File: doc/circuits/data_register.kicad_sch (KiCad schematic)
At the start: 12 parts, among them U1 74LS193, U10 74LS32, U11 74LS32, U13 74LS193, U2 74LS00, U3 74LS245, U4 74LS00, U5 74LS00, U6 74LS32, U7 74LS245, U8 74LS32, U9 74LS32

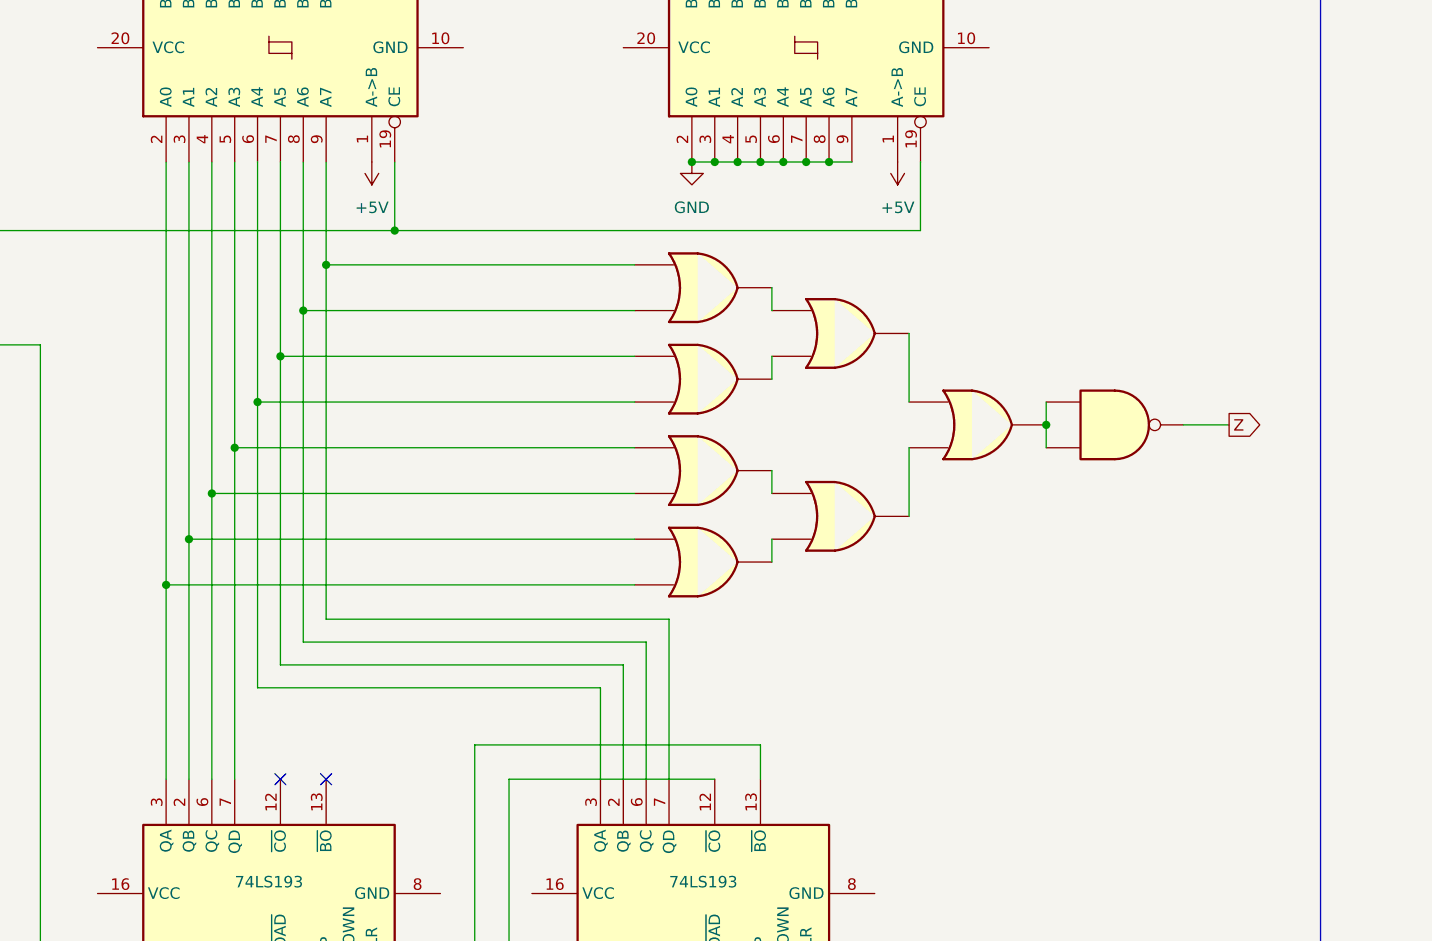
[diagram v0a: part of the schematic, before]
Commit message: more documentation
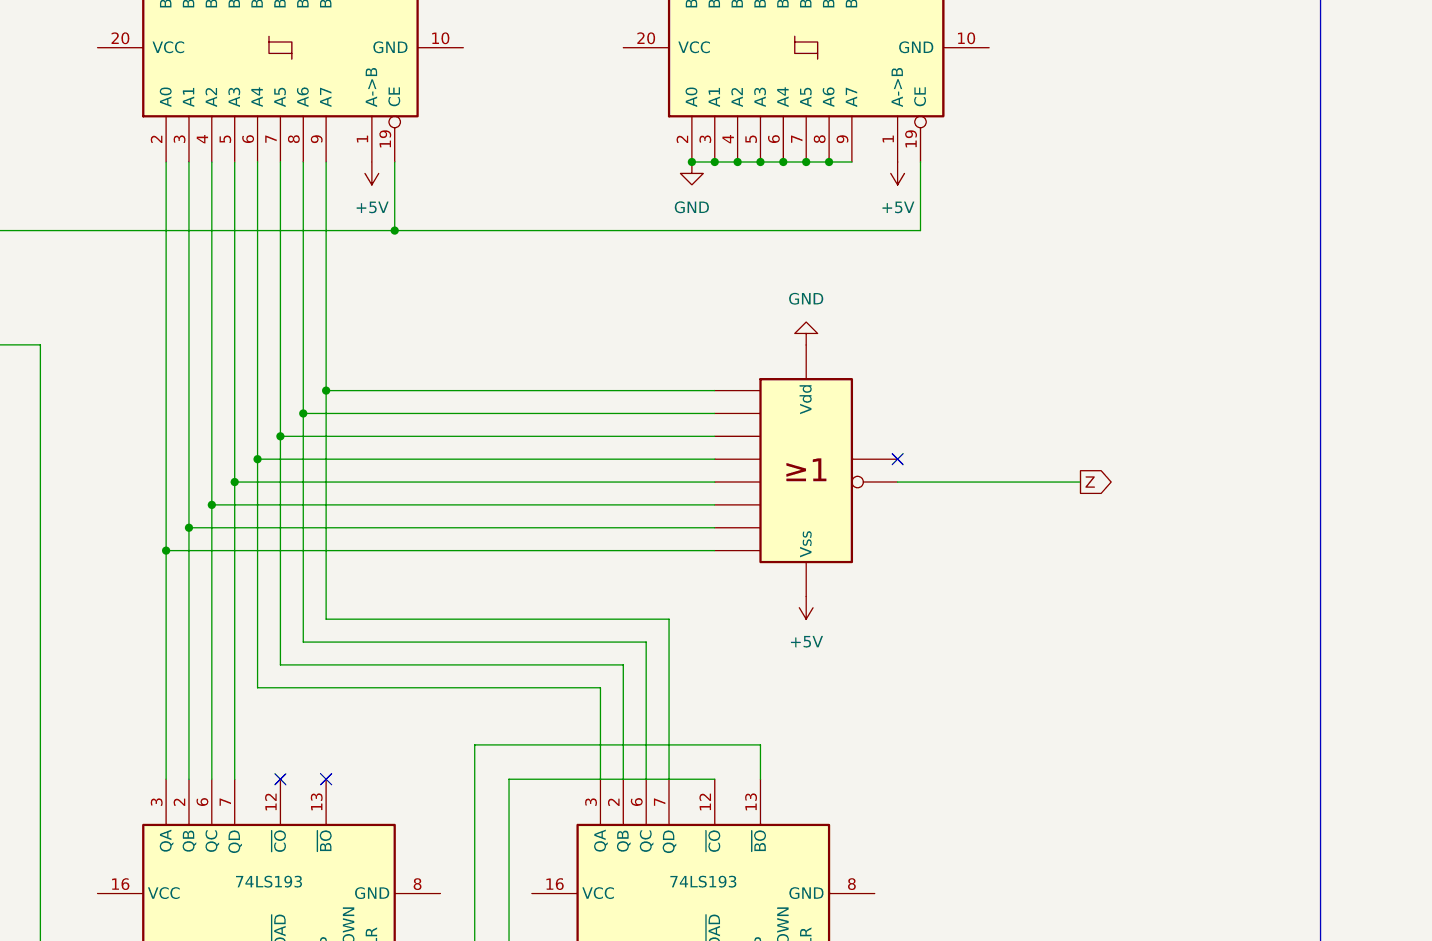
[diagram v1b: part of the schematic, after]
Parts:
- removed U10, U11, U6, U8, U9: 74LS32, symbol 74xx:74LS32
- removed U4: 74LS00, symbol 74xx:74LS00
- added U12: 4078, symbol 4xxx_IEEE:4078
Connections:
- net +5V: now also U12.7 (Vss)
- net GND: now also U12.14 (Vdd)
- net Z: now also U12.13
- net at U1.3 (QA), U3.2 (A0): now also U12.12
- net at U1.2 (QB), U3.3 (A1): now also U12.11
- net at U1.6 (QC), U3.4 (A2): now also U12.10
- net at U1.7 (QD), U3.5 (A3): now also U12.9
- net at U13.3 (QA), U3.6 (A4): now also U12.5
- net at U13.2 (QB), U3.7 (A5): now also U12.4
- net at U13.6 (QC), U3.8 (A6): now also U12.3
- net at U13.7 (QD), U3.9 (A7): now also U12.2
- no-connect marks 2 -> 3
